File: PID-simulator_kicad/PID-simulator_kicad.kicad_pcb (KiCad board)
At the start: 2 copper layers, 104.8 x 72.4 mm, 11 parts, among them SW1 Set, SW2 P, SW3 I, SW4 D, U1 L298N Module, U2 Motor, U3 GM009605_0.96"_OLED_Screen, U4 6V In

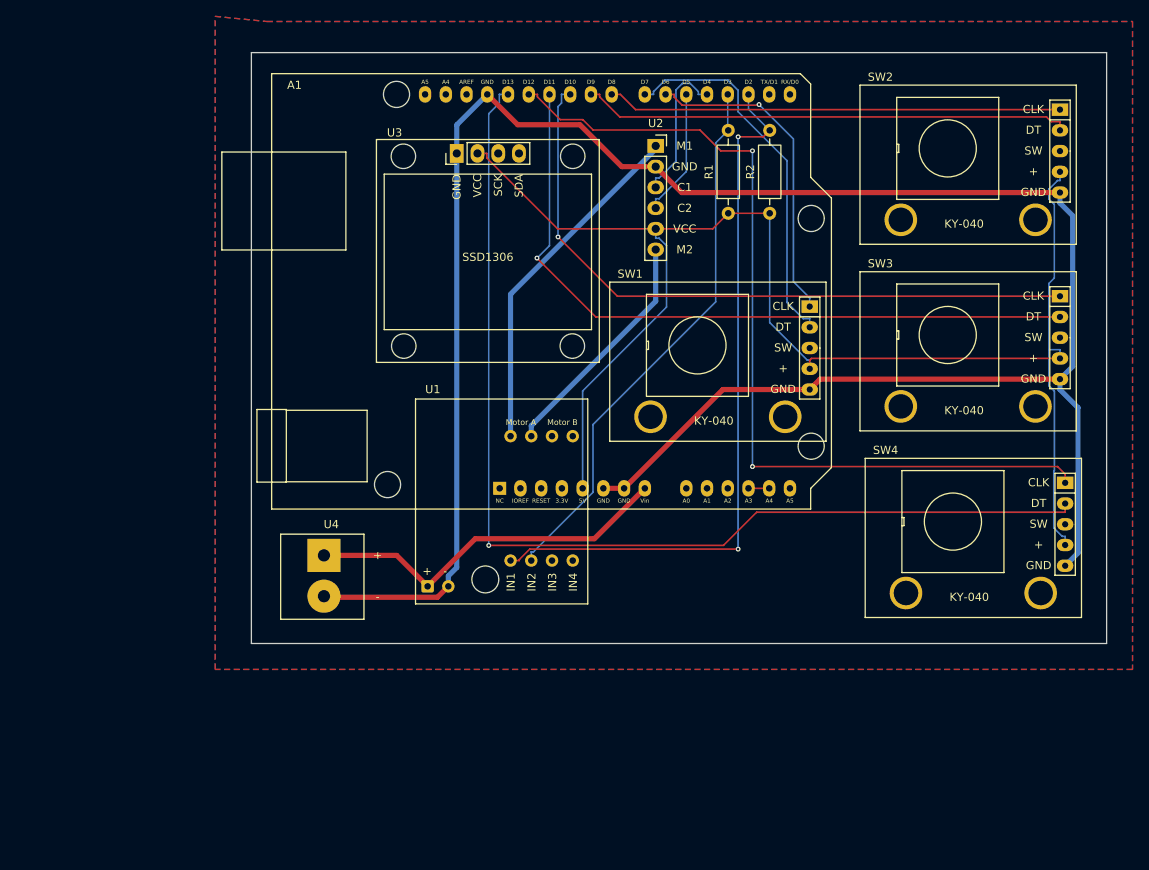
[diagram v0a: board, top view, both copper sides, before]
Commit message: pcb update
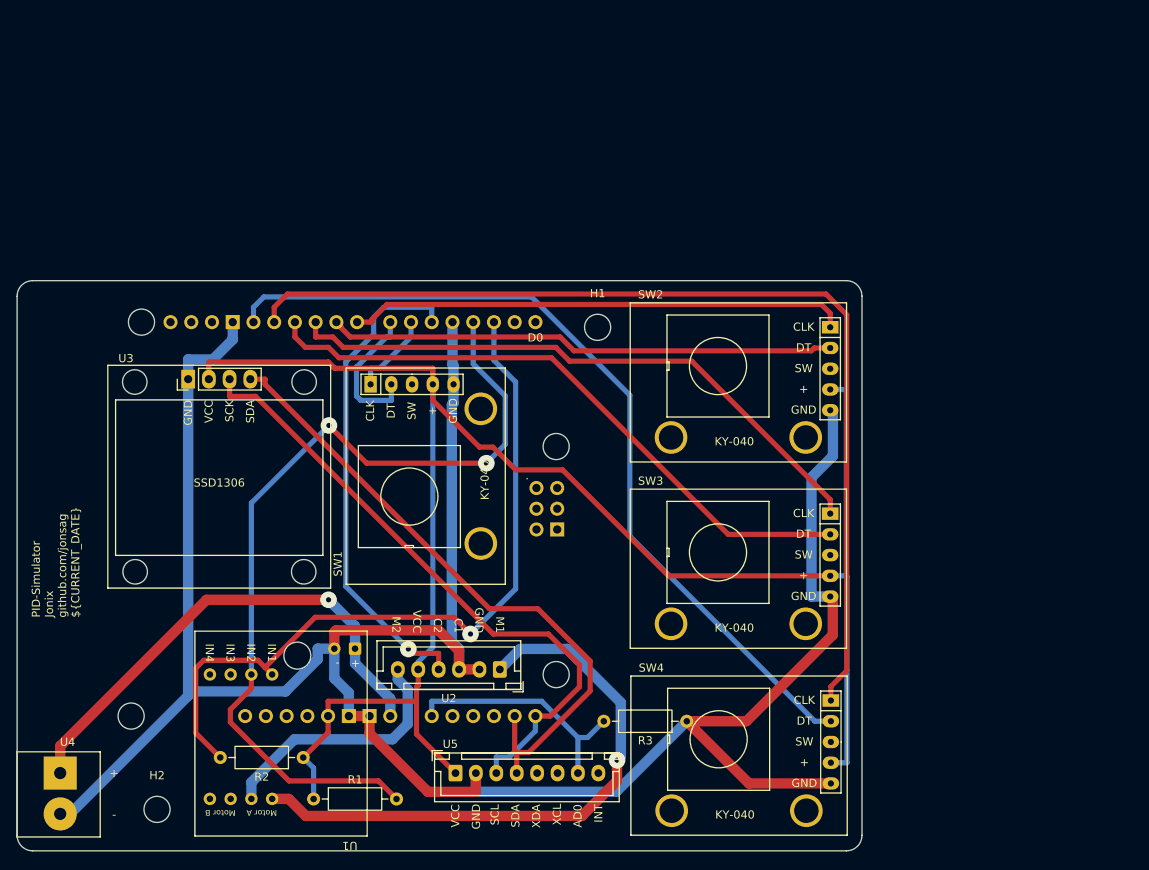
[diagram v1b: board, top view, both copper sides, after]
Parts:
- added H1: MountingHole, MountingHole:MountingHole_3.2mm_M3, F.Cu at (171.3, 63.5)
- added H2: MountingHole, MountingHole:MountingHole_3.2mm_M3, F.Cu at (117.3, 122.6)
- added R3: 10k, Resistor_THT:R_Axial_DIN0207_L6.3mm_D2.5mm_P10.16mm_Horizontal, F.Cu at (182.2, 111.8)
- added U5: GY-521_MPU6050_v2, MyFootprints:8-pin JST MPU6050, F.Cu at (153.9, 118.1)
- A1: footprint MyFootprints:Arduino_UNO_R3_shield_large -> PCM_arduino-library:Arduino_Uno_R3_Shield
- U2: footprint MyFootprints:6-pin N20 DC Motor w Encoder -> MyFootprints:6-pin JST N20 DC Motor w Encoder
- U3: value GM009605_0.96"_OLED_Screen -> GM009605 Screen
- moved R1 87.9 mm to (136.5, 121.3), turned to 0 degrees
- moved R2 87.8 mm to (135.3, 116.2), turned to 180 degrees
- moved A1 87.0 mm to (100.2, 113.7)
- moved U2 66.9 mm to (159.3, 105.4), turned to 180 degrees
- moved SW1 54.6 mm to (143.5, 70.5), turned to 90 degrees
- moved U3 43.0 mm to (121.2, 69.8)
- moved U4 41.9 mm to (105.5, 118.1)
- moved SW4 39.2 mm to (199.9, 109.2)
- moved SW2 38.8 mm to (199.8, 63.5)
- moved SW3 38.7 mm to (199.8, 86.3)
- moved U1 11.7 mm to (141.6, 102.9), turned to 180 degrees
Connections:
- net /D10 renamed /D10 - I CLK
- net /D11 renamed /D11 - I DT
- net /D12 renamed /D12 - D CLK
- net /D13 renamed /D13 - D DT
- net /D6 renamed /D6 - Set CLK
- net /D7 renamed /D7 - Set DT
- net /D8 renamed /D8 - P CLK
- net /D9 renamed /D9 - P DT
- A1 pad A0: unconnected-(A1-PadA0) -> Net-(U5-AD0)
- A1 pad A4: unconnected-(A1-PadA4) -> /SDA
- A1 pad A5: unconnected-(A1-PadA5) -> /SCL
- A1 pad D4: /D4 - C1 -> GND
- U2 pad 3: /D4 - C1 -> GND
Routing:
- net /SDA: track 0.00 -> 79.2 mm
- net /SCL: track 0.00 -> 78.1 mm
- net /D5 - C2: track 15.7 -> 60.6 mm, vias 0 -> 1
- net /D3 - IN2: track 67.3 -> 106.7 mm, vias 0 -> 2
- net +5V: track 181.2 -> 218.1 mm
- net GND: track 263.3 -> 296.5 mm
- net /MotorA-1: track 42.9 -> 73.3 mm, vias 0 -> 1
- net Net-(U5-AD0): track 0.00 -> 29.9 mm
- net /D6 - Set CLK: track 39.6 -> 10.3 mm, vias 1 -> 0
- net /D7 - Set DT: track 46.0 -> 17.5 mm
- net /D13 - D DT: track 130.2 -> 104.7 mm, vias 1 -> 0
- net /D4 - C1: track 18.1 -> 0.00 mm
- net +6V: track 45.9 -> 61.0 mm, vias 0 -> 1
- net /D12 - D CLK: track 108.9 -> 121.7 mm, vias 2 -> 0
- net /D11 - I DT: track 87.7 -> 77.4 mm, vias 1 -> 0
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- removed copper zone on B.Cu, net GND
- removed copper zone on F.Cu, net GND
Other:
- board size 104.8 x 72.4 mm -> 103.5 x 69.9 mm
- board text added: "${TITLE} ${COMPANY} github.com/jonsag ${CURRENT_DATE}"
